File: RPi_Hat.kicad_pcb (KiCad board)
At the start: 2 copper layers, 65 x 56.5 mm, 22 parts, among them IC1 0.96_I2C_OLED, IC2 7406, IC3 I2C LC, IC4 0.96_I2C_OLED, J1 RPi_GPIO, SW1 Select, SW2 Up, SW3 Down, SW4 Exit, SW5 Add Disk

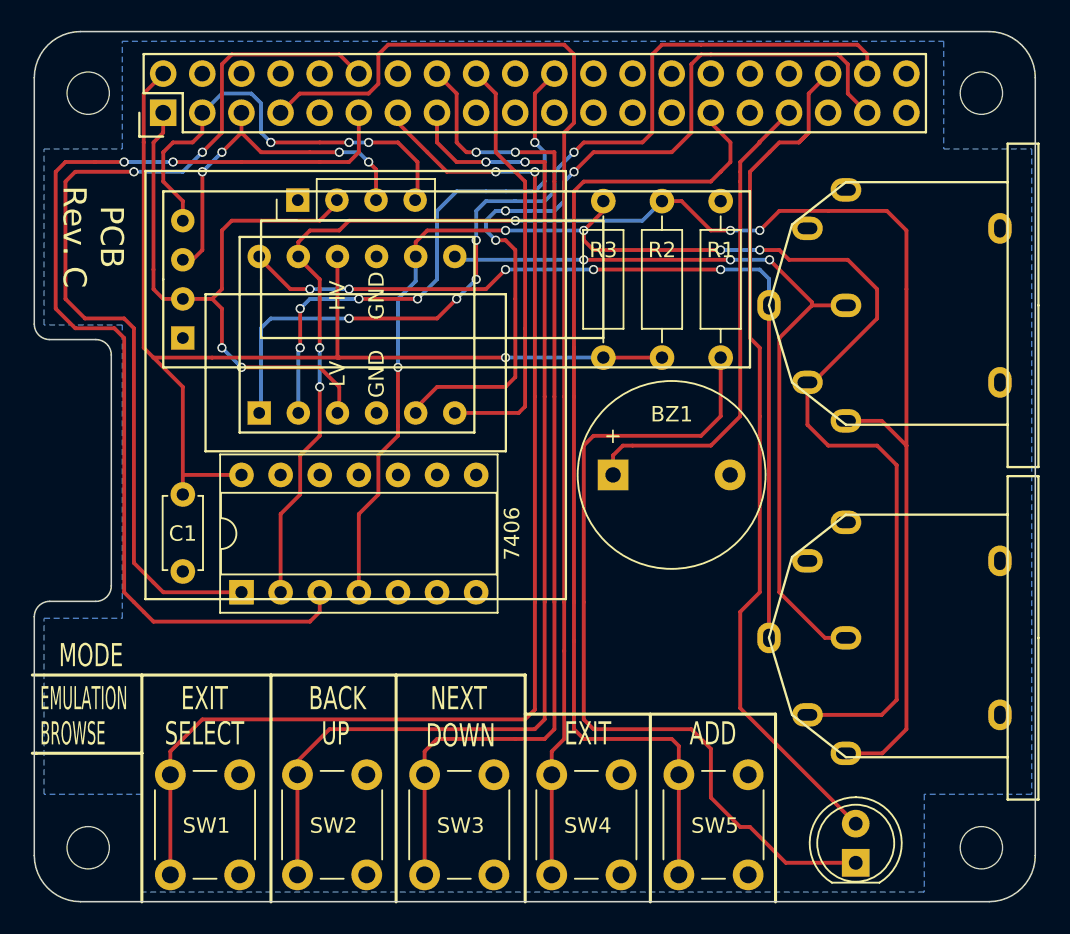
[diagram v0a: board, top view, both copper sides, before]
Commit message: pi1551 hat, test version (20251022)
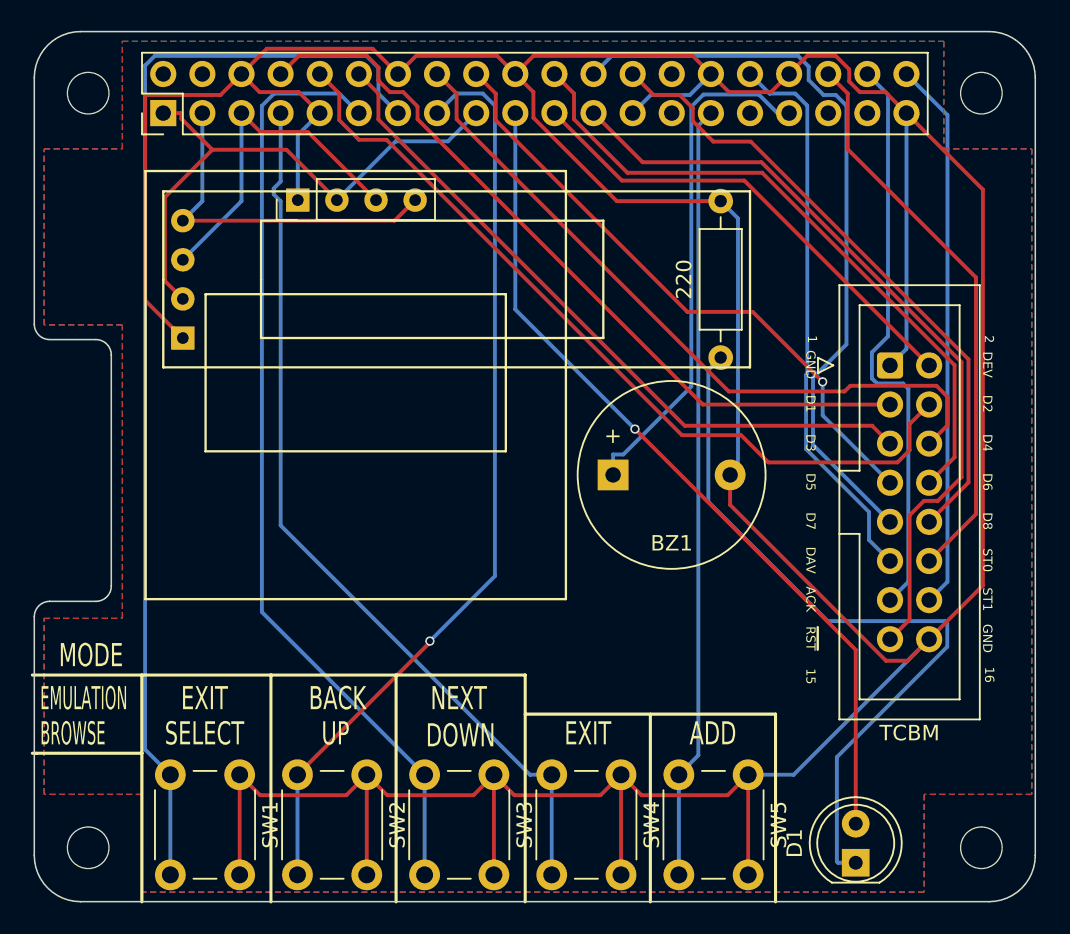
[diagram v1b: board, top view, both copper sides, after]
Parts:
- removed ? (x4): , RPi_Hat:RPi_Hat_Mounting_Hole
- removed C1: 100nF, Capacitors_THT:C_Disc_D4.7mm_W2.5mm_P5.00mm
- removed IC2: 7406, Housings_DIP:DIP-14_W7.62mm_Socket
- removed IC3: I2C LC, IIC_4CH_Level_Converter:4CH_I2C_Level_Converter
- removed IEC_1, IEC_2: C64_IEC, C64_IEC:C64_IEC
- removed R2, R3: 1K, Resistors_THT:R_Axial_DIN0207_L6.3mm_D2.5mm_P10.16mm_Horizontal
- added H1: MountingHole, MountingHole:MountingHole_2.7mm_M2.5_DIN965, F.Cu at (85.0, 32.6)
- added H2: MountingHole, MountingHole:MountingHole_2.7mm_M2.5_DIN965, F.Cu at (27.0, 32.6)
- added H3: MountingHole, MountingHole:MountingHole_2.7mm_M2.5_DIN965, F.Cu at (85.0, 81.6)
- added H4: MountingHole, MountingHole:MountingHole_2.7mm_M2.5_DIN965, F.Cu at (27.0, 81.6)
- added J2: TCBM, Connector_IDC:IDC-Header_2x08_P2.54mm_Vertical, F.Cu at (79.1, 50.3)
- BZ1: footprint Buzzers_Beepers:Buzzer_12x9.5RM7.6 -> Buzzer_Beeper:Buzzer_12x9.5RM7.6
- D1: footprint LEDs:LED_D5.0mm -> LED_THT:LED_D5.0mm
- J1: footprint RPi_Hat:Pin_Header_Straight_2x20 -> Connector_PinHeader_2.54mm:PinHeader_2x20_P2.54mm_Vertical
- R1: value 100 -> 220; footprint Resistors_THT:R_Axial_DIN0207_L6.3mm_D2.5mm_P10.16mm_Horizontal -> Resistor_THT:R_Axial_DIN0207_L6.3mm_D2.5mm_P10.16mm_Horizontal
- SW1, SW2, SW3, SW4, SW5: footprint Buttons_Switches_THT:SW_PUSH_6mm_h5mm -> Button_Switch_THT:SW_PUSH_6mm_H5mm
- moved J1 24.2 mm to (31.9, 33.9)
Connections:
- net I2C_SCL renamed /I2C_SCL
- net I2C_SDA renamed /I2C_SDA
- net IN_SW1 renamed /IN_SW1
- net IN_SW2 renamed /IN_SW2
- net IN_SW4 renamed /IN_SW4
- net IN_SW5 renamed /IN_SW5
- net RPI_SND renamed /RPI_SND
- D1 pad 2: RPI_LED -> /RPI_LED
- J1 pad 10: (no net) -> /DIO2
- J1 pad 11: RPI_CLK_OUT -> /IN_SW3
- J1 pad 12: RPI_DATA_OUT -> /DIO3
- J1 pad 16: IN_SW3 -> /DIO4
- J1 pad 17: (no net) -> +3V3
- J1 pad 18: RPI_ATN -> /DIO5
- J1 pad 19: (no net) -> /RPI_LED
- J1 pad 2: +5V -> unconnected-(J1-5V-Pad2)
- J1 pad 21: (no net) -> /DEV
- J1 pad 22: RPI_DATA_IN -> /DIO6
- J1 pad 23: (no net) -> /~{RESET}
- J1 pad 24: (no net) -> /DIO7
- J1 pad 26: (no net) -> /DIO8
- J1 pad 27: (no net) -> unconnected-(J1-BCM0_ID_SD-Pad27)
- J1 pad 28: (no net) -> unconnected-(J1-BCM1_ID_SC-Pad28)
- J1 pad 31: (no net) -> unconnected-(J1-BCM6-Pad31)
- J1 pad 32: (no net) -> /DAV
- J1 pad 35: (no net) -> unconnected-(J1-BCM19_MISO-Pad35)
- J1 pad 36: RPI_LED -> /STATUS0
- J1 pad 37: RPI_CLK_IN -> unconnected-(J1-BCM26-Pad37)
- J1 pad 38: RPI_RST -> /ACK
- J1 pad 4: (no net) -> unconnected-(J1-5V-Pad4)
- J1 pad 40: (no net) -> /STATUS1
- J1 pad 8: (no net) -> /DIO1
- SW3 pad 2: IN_SW3 -> /IN_SW3
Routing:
- net GND: track 0.00 -> 287.7 mm
- net C64_DATA: track 108.4 -> 0.00 mm, vias 5 -> 0
- net C64_CLK: track 98.2 -> 0.00 mm, vias 5 -> 0
- net +5V: track 72.4 -> 0.00 mm, vias 1 -> 0
- net RPI_CLK_OUT: track 69.1 -> 0.00 mm, vias 2 -> 0
- net IN_SW3: track 66.1 -> 0.00 mm, vias 2 -> 0
- net /IN_SW3: track 0.00 -> 61.5 mm
- net RPI_DATA_OUT: track 61.5 -> 0.00 mm, vias 2 -> 0
- net RPI_RST: track 60.4 -> 0.00 mm, vias 5 -> 0
- net C64_RST: track 58.1 -> 0.00 mm, vias 5 -> 0
- net RPI_LED: track 56.3 -> 0.00 mm
- net /RPI_LED: track 0.00 -> 55.3 mm, vias 0 -> 1
- net RPI_CLK_IN: track 54.2 -> 0.00 mm, vias 3 -> 0
- net /DIO2: track 0.00 -> 53.6 mm
- net C64_ATN: track 51.9 -> 0.00 mm, vias 3 -> 0
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- added copper zone on F.Cu, net GND
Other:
- net class Default removed
- board text added: "1"
- board text added: "15"
- board text added: "16"
- board text added: "2"
- board text added: "ACK"
- board text added: "D1"
- board text added: "D2"
- board text added: "D3"
- board text added: "D4"
- board text added: "D5"
- board text added: "D6"
- board text added: "D7"
- board text added: "D8"
- board text added: "DAV"
- board text added: "DEV"
- board text added: "GND"
- board text added: "Maciej Witkowiak <ytm@elysium.pl>, X 2025"
- board text added: "Pi1551"
- board text added: "ST0"
- board text added: "ST1"
- board text added: "~{RST}"
- board text removed: "PCB Rev. C"
- board text removed: "Pi1541"
- board text removed: "https://hvetebolle.blogspot.com"
